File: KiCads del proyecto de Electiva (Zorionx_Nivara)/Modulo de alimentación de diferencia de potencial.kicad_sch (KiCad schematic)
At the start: 14 parts, among them U1 AP63203WU

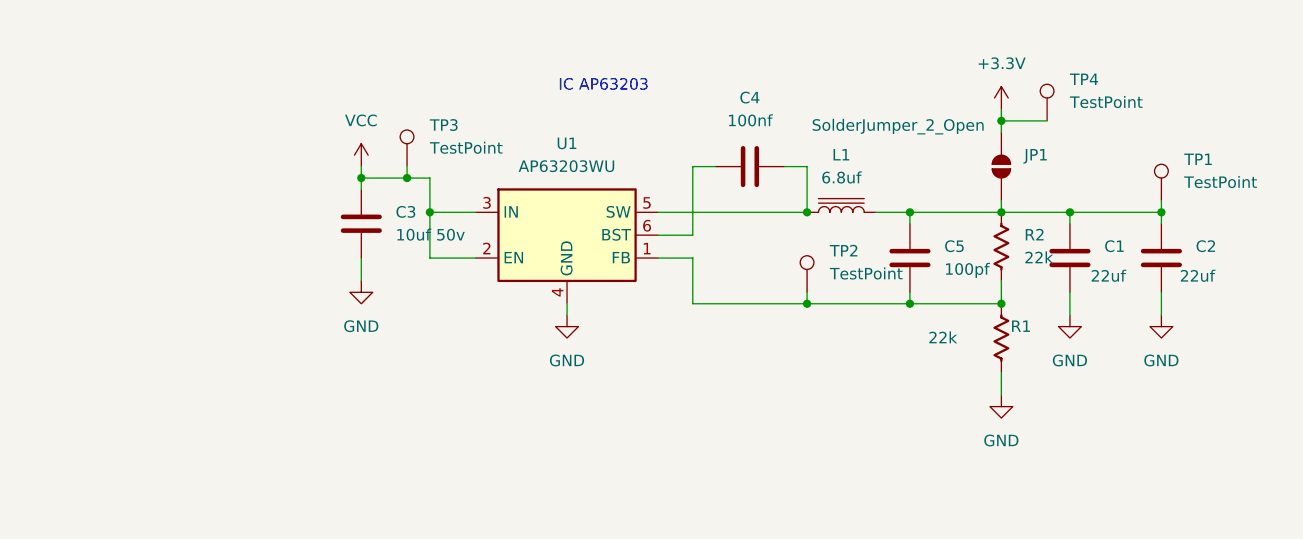
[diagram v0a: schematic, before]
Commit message: Esquemas PCB Readys
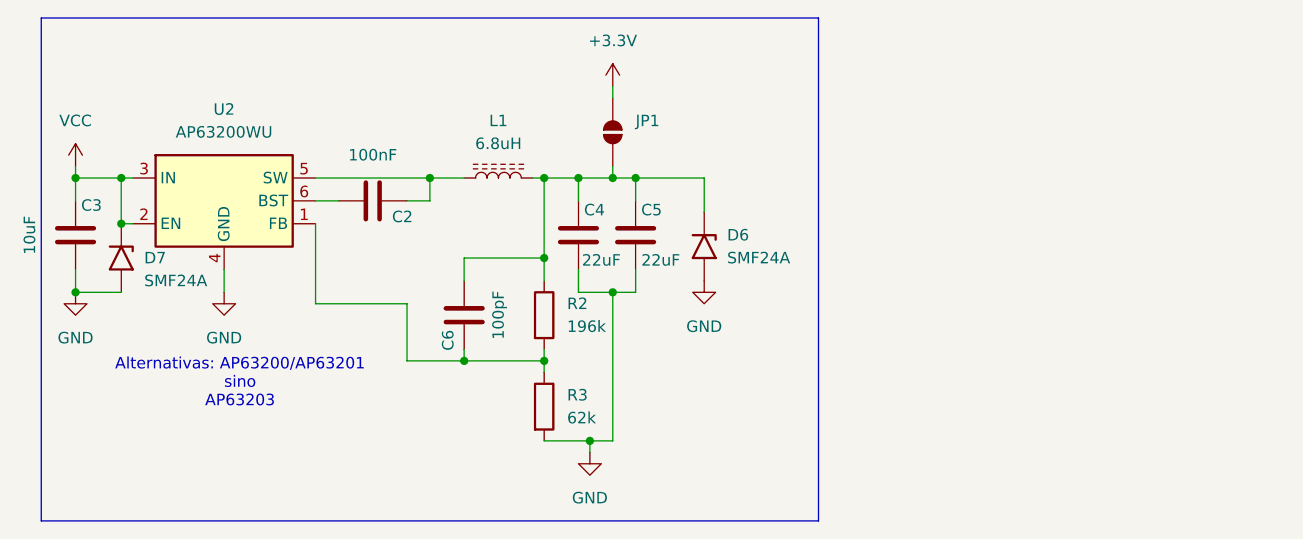
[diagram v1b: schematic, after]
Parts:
- removed C1: 22uf, Capacitor_SMD:C_0603_1608Metric_Pad1.08x0.95mm_HandSolder, symbol Device:C
- removed L1: 6.8uf, Inductor_SMD:L_Chilisin_BMRA00040420, symbol Device:L_Iron
- removed R1, R2: 22k, PCM_Resistor_SMD_AKL:R_0402_1005Metric, symbol PCM_Resistor_US_AKL:R_0402
- removed TP1, TP2, TP3, TP4: TestPoint, PCM_4ms_TestPoint:TestPoint_WireHole, symbol PCM_4ms_Connector:TestPoint
- removed U1: AP63203WU, Package_TO_SOT_SMD:TSOT-23-6, symbol Regulator_Switching:AP63203WU
- added C6: 100pF, symbol Device:C
- added D6, D7: SMF24A, Diode_SMD:D_SMF, symbol Diode:SMF24A
- added L1: 6.8uH, symbol Device:L_Ferrite
- added R2: 196k, symbol Device:R
- added R3: 62k, symbol Device:R
- added U2: AP63200WU, Package_TO_SOT_SMD:TSOT-23-6, symbol Regulator_Switching:AP63200WU
- C2: value 22uf -> 100nF; footprint Capacitor_SMD:C_0603_1608Metric_Pad1.08x0.95mm_HandSolder -> (none)
- C3: value 10uf 50v -> 10uF; footprint Capacitor_SMD:C_1206_3216Metric_Pad1.33x1.80mm_HandSolder -> (none); Voltage (none) -> 50V
- C4: value 100nf -> 22uF; footprint Capacitor_SMD:C_0603_1608Metric -> (none)
- C5: value 100pf -> 22uF; footprint Capacitor_SMD:C_0603_1608Metric_Pad1.08x0.95mm_HandSolder -> (none)
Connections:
- net +3.3V: now also JP1.2 (B); no longer JP1.1 (A)
- net GND: now also C3.1, C4.1, C5.1, D6.2 (A2), D7.2 (A2), R3.2, U2.4 (GND); no longer C2.2, C3.2
- net VCC: now also C3.2, D7.1 (A1), U2.2 (EN), U2.3 (IN); no longer C3.1
- net at C5.2: now also C4.2, JP1.1 (A), C6.1, D6.1 (A1), L1.2, R2.1
- new net: C6.2, R2.2, R3.1, U2.1 (FB)
- new net: C2.2, L1.1, U2.5 (SW)
- new net: C2.1, U2.6 (BST)
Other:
- note added: "Alternativas: AP63200/AP63201 sino AP63203"
- note removed: "IC AP63203"
